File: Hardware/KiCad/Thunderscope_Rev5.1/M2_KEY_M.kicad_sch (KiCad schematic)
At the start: 46 parts, among them J1 BNC, J10 009155002852006, J11 7793, J2 BNC, J8 M.2 Key M, U17 TPS61023

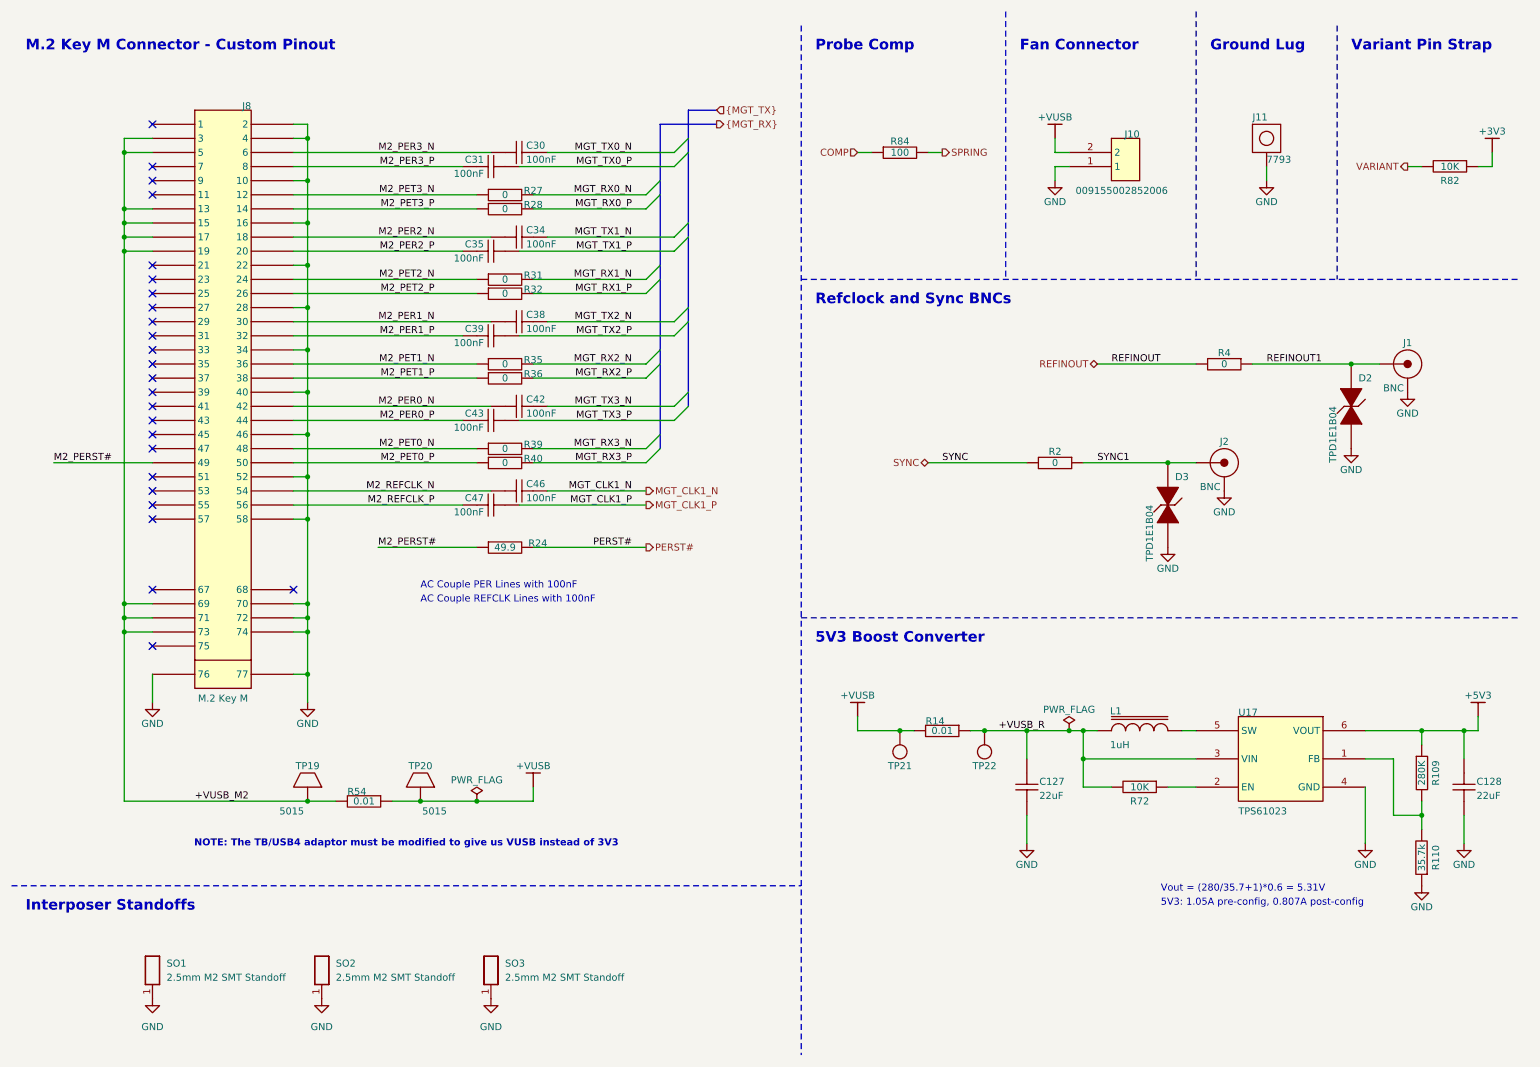
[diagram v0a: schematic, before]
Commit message: Added extra caps to boost reg - closes #336
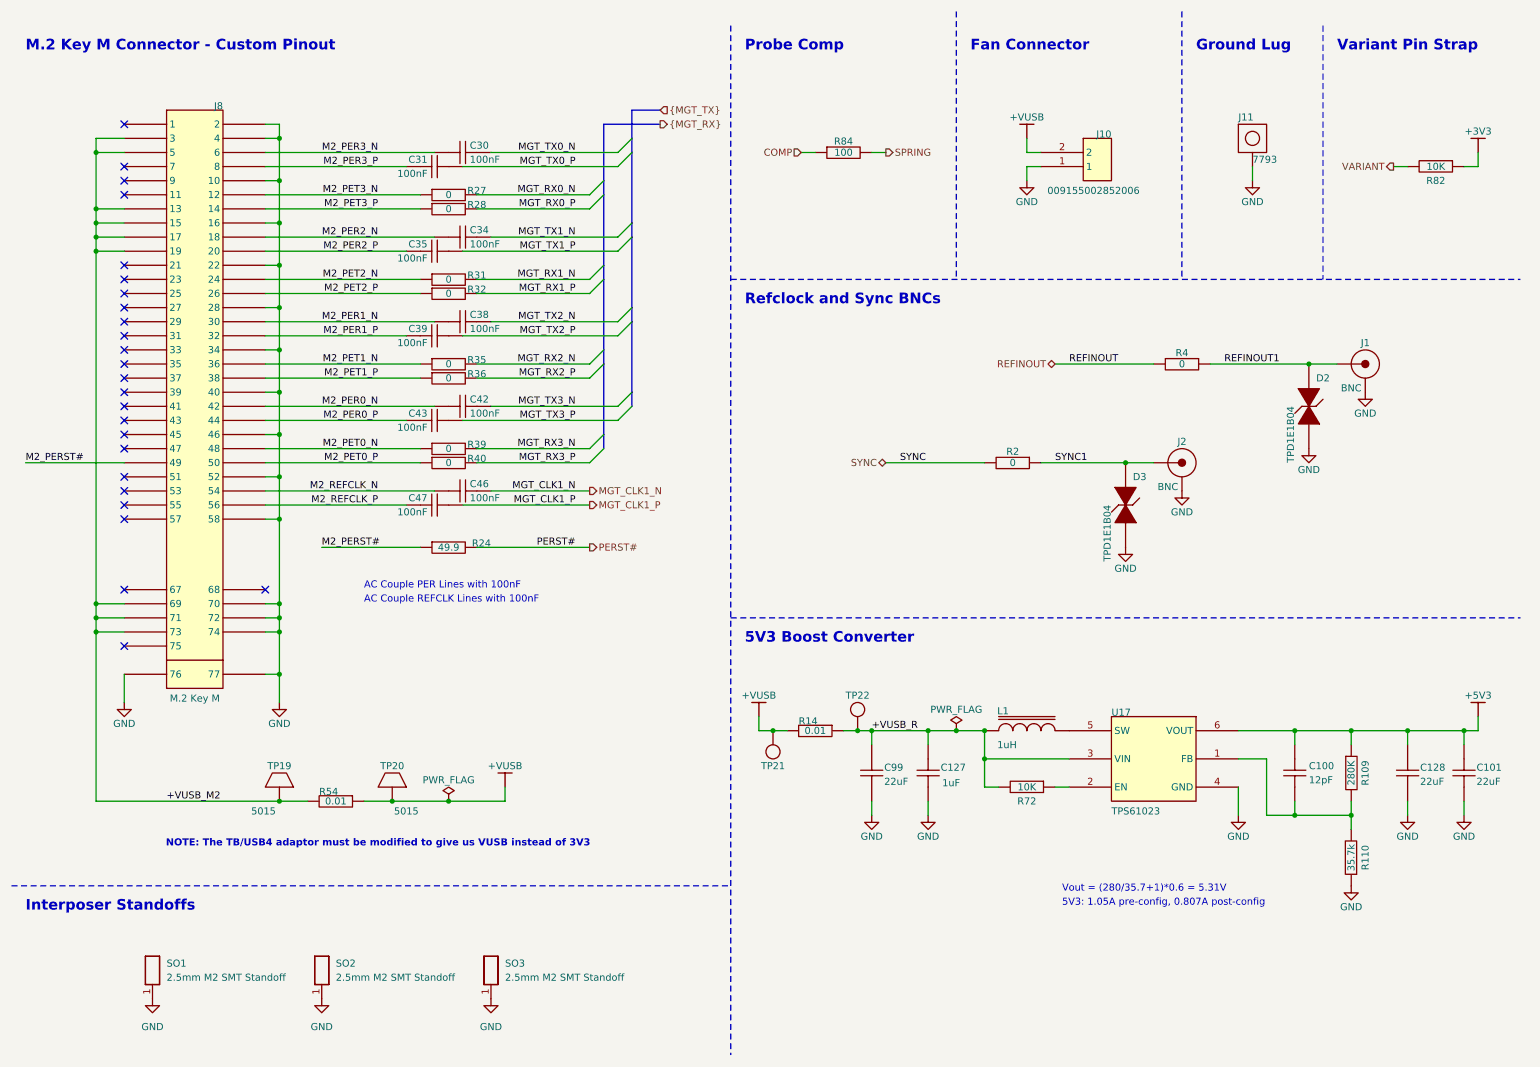
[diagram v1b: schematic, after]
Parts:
- added C100: 12pF, Thunderscope_Rev5:GEN_C_0402, symbol Thunderscope_Rev5:CAP 12pF 50V C0G 0402
- added C101, C99: 22uF, Thunderscope_Rev5:GEN_C_0805, symbol Thunderscope_Rev5:CAP 22uF 25V X5R 0805
- C127: value 22uF -> 1uF; footprint Thunderscope_Rev5:GEN_C_0805 -> Thunderscope_Rev5:GEN_C_0402; symbol Thunderscope_Rev5:CAP 22uF 25V X5R 0805 -> Thunderscope_Rev5:CAP 1uF 25V X5R 0402; HOUSE PART NUMBER C-22uF-0805-002 -> (none); MANUFACTURER PART NUMBER GRM21BR61E226ME44L -> GRM155R61E105KA12D; PACKAGE 0805 -> 0402; SUPPLIER PART NUMBER 1 81-GRM21BR61E226ME4L -> 81-GRM155R61E105KA2D
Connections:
- net +5V3: now also C100.2, C101.2
- net +VUSB_R: now also C127.1, C99.2; no longer C127.2
- net GND: now also C127.2, C101.1, C99.1; no longer C127.1
- net at R109.1, R110.1, U17.1 (FB): now also C100.1
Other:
- moved on the sheet: C127, C128, C30, C31, C34, C35, C38, C39, C42, C43, C46, C47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
